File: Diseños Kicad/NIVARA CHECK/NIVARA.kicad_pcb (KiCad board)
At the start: 2 copper layers, 107 x 87.7 mm, 41 parts, among them J1 Screw_Terminal_01x02, J10 Screw_Terminal_01x02, J12 Screw_Terminal_01x04, J2 Screw_Terminal_01x02, J3 Screw_Terminal_01x04, J4 Screw_Terminal_01x02, J5 Screw_Terminal_01x02, J6 Screw_Terminal_01x06, J7 Screw_Terminal_01x03, J9 Screw_Terminal_01x02, K1 G2RL-1, K2 G2RL-1, Q1 NCV8402xST, Q3 NCV8402xST, Q4 NCV8402xST, Q5 NCV8402xST, U1 ESP32-S3-WROOM-1, U10 LTV-357TB, U12 LTV-357T, U13 LTV-357T, U14 LTV-357T, U15 LTV-357TB, U2 AP63200WU, U2 AP63203WU, U4 LTV-357TB, U5 LTV-357T, U7 LTV-357TB, U8 LTV-357TB, U9 LTV-357TB

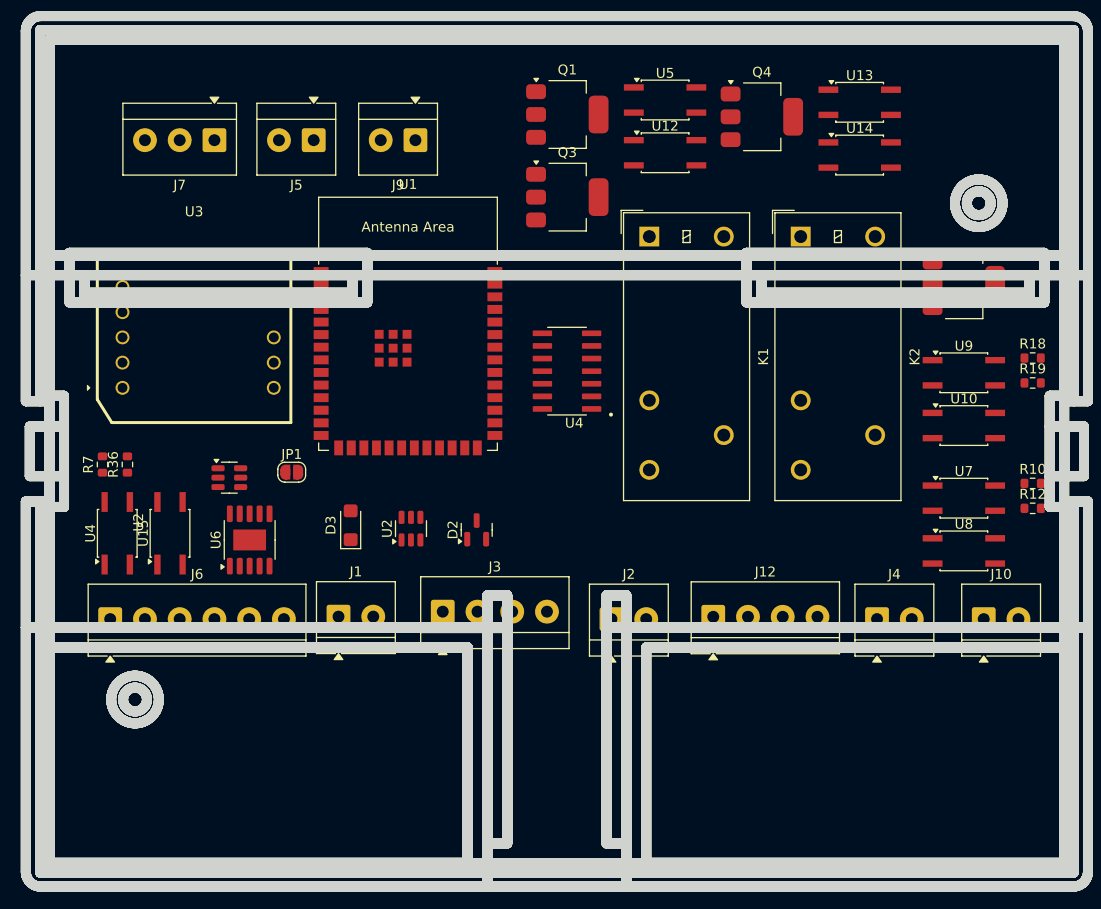
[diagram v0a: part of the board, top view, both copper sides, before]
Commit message: detallitos
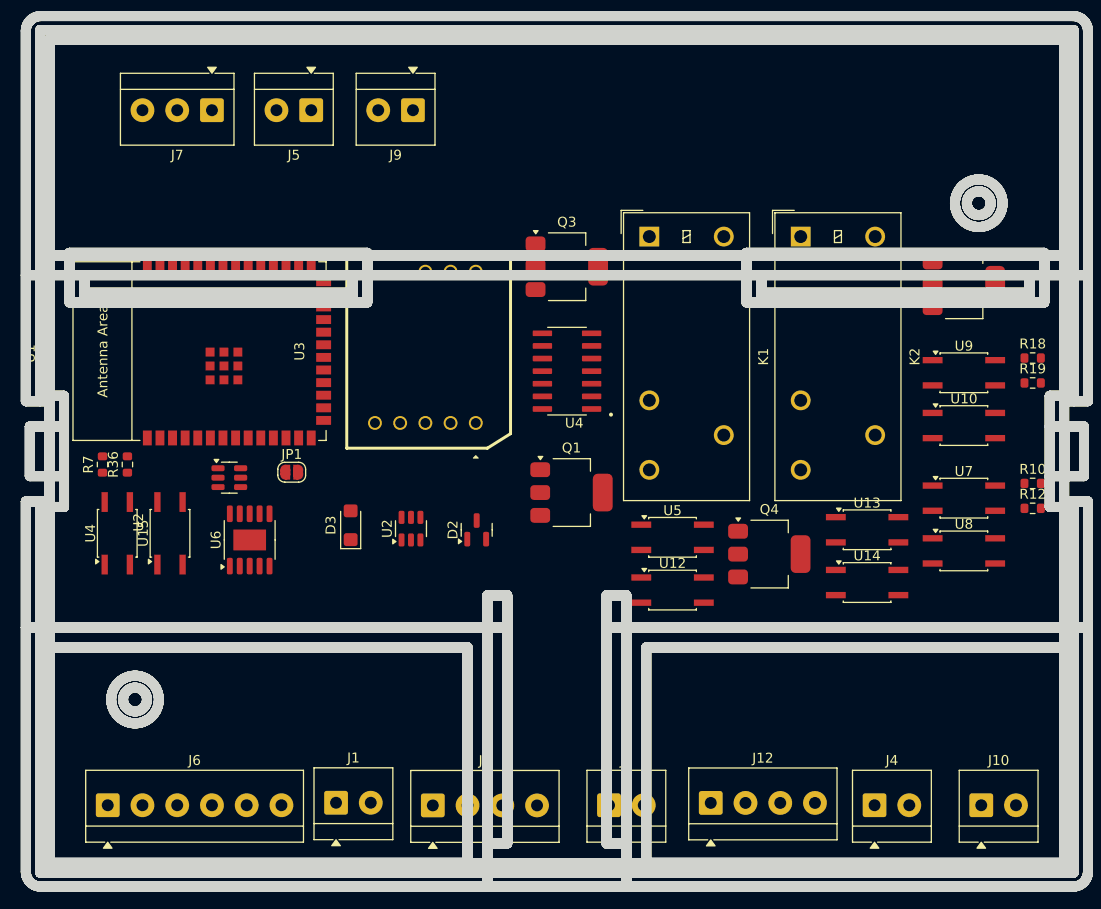
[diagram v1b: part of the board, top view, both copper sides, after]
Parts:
- moved U5 44.1 mm to (165.2, 83.0)
- moved Q4 44.1 mm to (174.9, 84.7)
- moved U12 44.1 mm to (165.2, 88.3)
- moved U13 43.1 mm to (184.8, 82.2)
- moved U14 43.1 mm to (184.8, 87.6)
- moved U3 41.7 mm to (148.8, 74.0), turned to 90 degrees
- moved Q1 38.1 mm to (155.0, 78.5)
- moved J3 19.5 mm to (141.0, 110.0)
- moved J1 18.8 mm to (131.2, 109.8)
- moved J10 18.8 mm to (196.2, 110.0)
- moved J12 18.8 mm to (169.0, 109.8)
- moved J2 18.8 mm to (158.8, 110.0)
- moved J4 18.8 mm to (185.5, 110.0)
- moved J6 18.8 mm to (108.2, 110.0)
- moved U1 18.0 mm to (120.5, 64.2), turned to 90 degrees
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
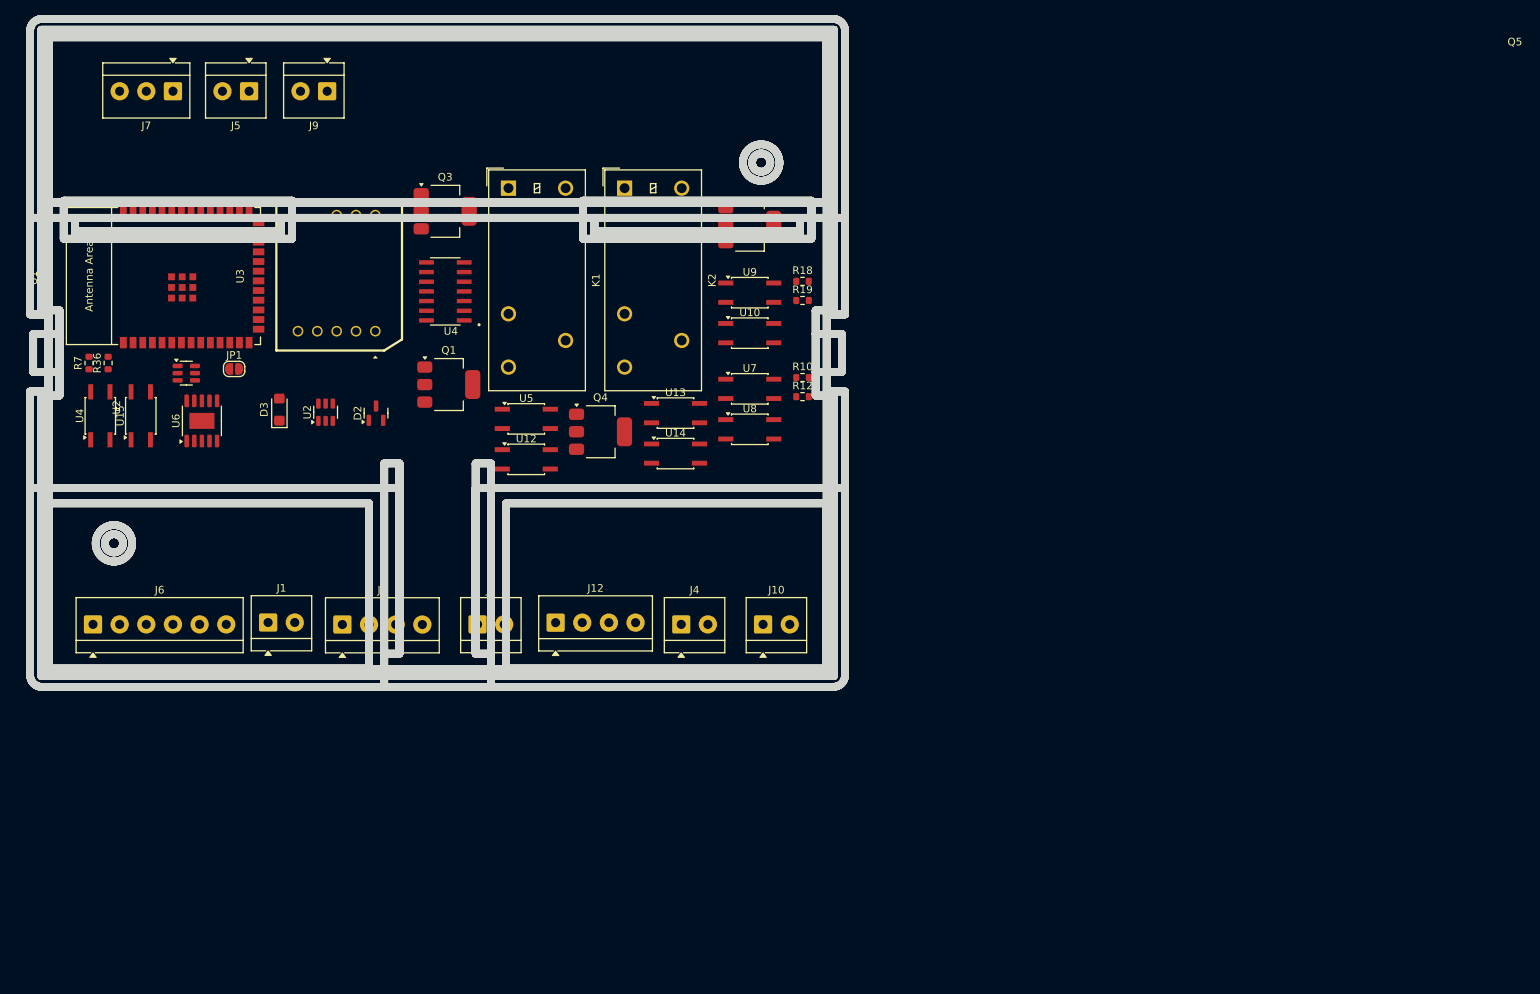
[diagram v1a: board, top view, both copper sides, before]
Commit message: YA AAAAAAAAAAAAAAAA
Detallitos sobre el dxf que estaba mal
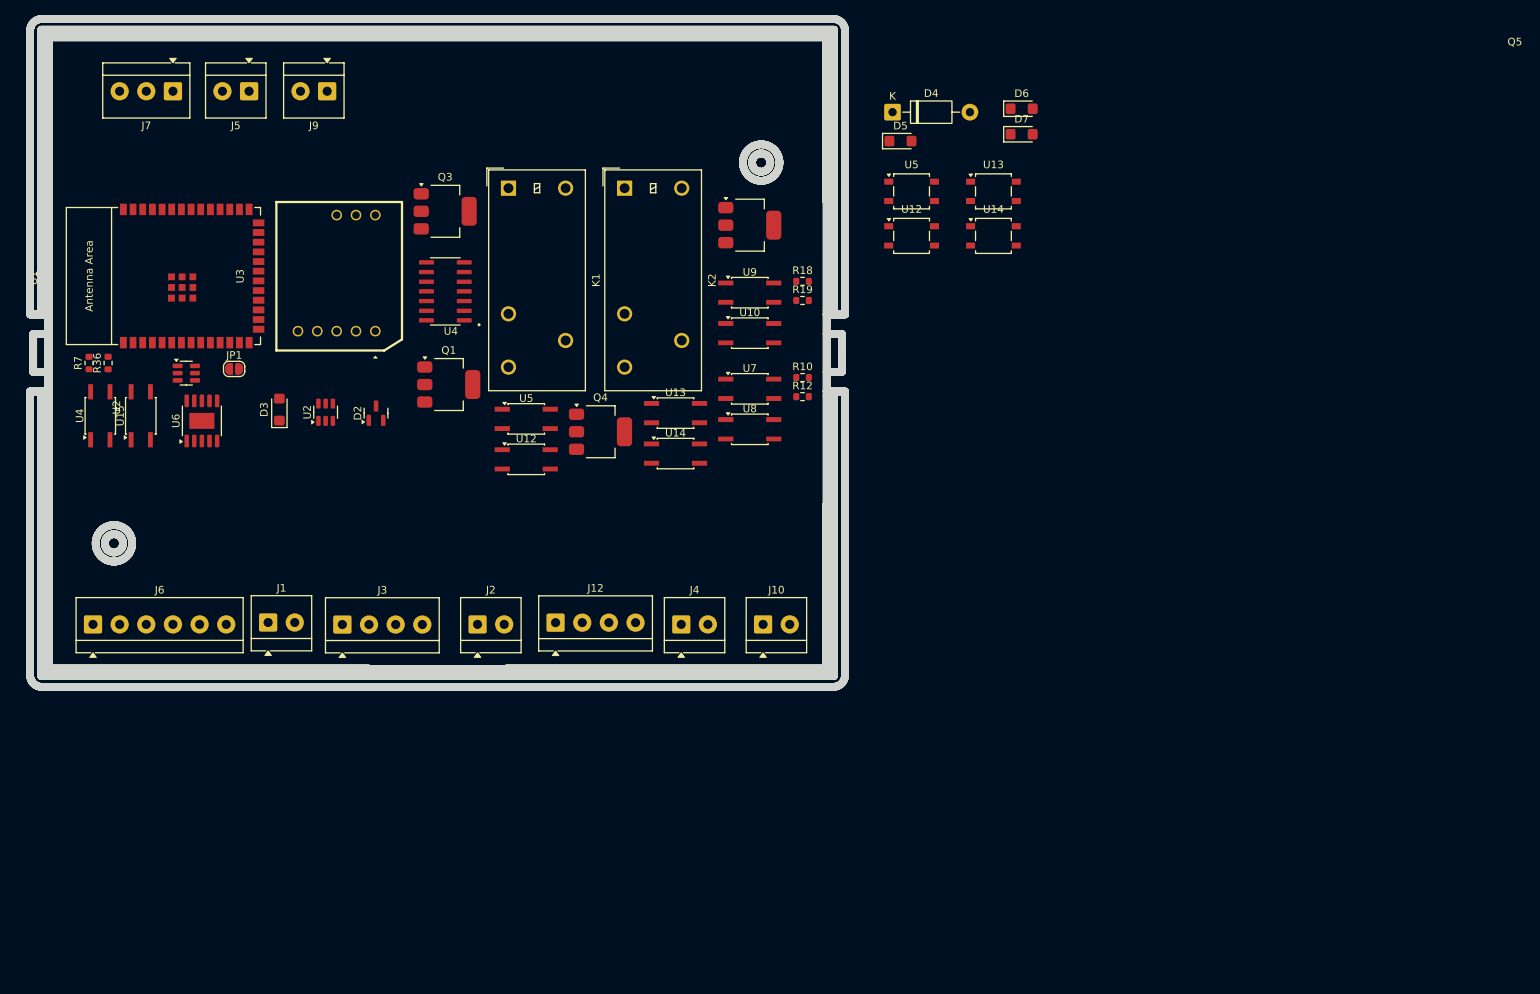
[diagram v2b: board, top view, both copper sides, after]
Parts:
- added D4: 1N4007, Diode_THT:D_DO-41_SOD81_P10.16mm_Horizontal, F.Cu at (213.2, 42.7)
- added D5: SMF24A, Diode_SMD:D_SMF, F.Cu at (214.3, 46.5)
- added D6: SMF24A, Diode_SMD:D_SMF, F.Cu at (230.2, 42.3)
- added D7: SMF24A, Diode_SMD:D_SMF, F.Cu at (230.2, 45.6)
- added U12: ~, Package_SO:SO-4_4.4x4.3mm_P2.54mm, F.Cu at (215.8, 59.0)
- added U13: ~, Package_SO:SO-4_4.4x4.3mm_P2.54mm, F.Cu at (226.5, 53.1)
- added U14: ~, Package_SO:SO-4_4.4x4.3mm_P2.54mm, F.Cu at (226.5, 59.0)
- added U5: ~, Package_SO:SO-4_4.4x4.3mm_P2.54mm, F.Cu at (215.8, 53.1)
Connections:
- J12 pad 3: /NIVARA_BOARD/mA_AOUTPUT- -> unconnected-(J12-Pin_3-Pad3)
- J6 pad 1: /NIVARA_BOARD/RL1_COM -> /NIVARA_BOARD/RL1_OUTPUT_NO
- J6 pad 5: /NIVARA_BOARD/RL1_COM -> /NIVARA_BOARD/RL2_OUTPUT_NC
- JP1 pad 1: Net-(JP1-A) -> Net-(D6-A1)
- K1 pad 12: /NIVARA_BOARD/RL1_COM -> /NIVARA_BOARD/RL2_OUTPUT_NC
- K2 pad 14: /NIVARA_BOARD/RL1_COM -> /NIVARA_BOARD/RL1_OUTPUT_NO
- U1 pad 12: unconnected-(U1-GPIO8/TOUCH8/ADC1_CH7/SUBSPICS1-Pad12) -> /NIVARA_BOARD/PNP_IN_Mod/NPN_Output0
- U1 pad 16: unconnected-(U1-GPIO46-Pad16) -> /NIVARA_BOARD/~{TRANSMIT}/RECEIVE
- U1 pad 17: unconnected-(U1-GPIO9/TOUCH9/ADC1_CH8/FSPIHD/SUBSPIHD-Pad17) -> /NIVARA_BOARD/PNP_IN_Mod/NPN_Output1
- U1 pad 18: unconnected-(U1-GPIO10/TOUCH10/ADC1_CH9/FSPICS0/FSPIIO4/SUBSPICS0-Pad18) -> /NIVARA_BOARD/DRY_INPUT_INTERFAZ/DRY_OUT0
- U1 pad 23: unconnected-(U1-GPIO21-Pad23) -> /NIVARA_BOARD/DRY_INPUT_INTERFAZ/DRY_OUT1
- U1 pad 24: unconnected-(U1-GPIO47/SPICLK_P/SUBSPICLK_P_DIFF-Pad24) -> /NIVARA_BOARD/RS485_INTERFAZ/UART_TX
- U1 pad 25: unconnected-(U1-GPIO48/SPICLK_N/SUBSPICLK_N_DIFF-Pad25) -> /NIVARA_BOARD/RS485_INTERFAZ/UART_RX
- U1 pad 26: unconnected-(U1-GPIO45-Pad26) -> /NIVARA_BOARD/NPN_OUT_INTERFAZ/NPN_EN1
- U1 pad 28: unconnected-(U1-SPIIO6/GPIO35/FSPID/SUBSPID-Pad28) -> /NIVARA_BOARD/VOLTAGE_AOUT_INTERFAZ/SEL
- U1 pad 29: unconnected-(U1-SPIIO7/GPIO36/FSPICLK/SUBSPICLK-Pad29) -> /NIVARA_BOARD/~{RUN}/STOP
- U1 pad 31: unconnected-(U1-GPIO38/FSPIWP/SUBSPIWP-Pad31) -> /NIVARA_BOARD/NPN_OUT_INTERFAZ/NPN_EN0
- U1 pad 36: /NIVARA_BOARD/RS485_INTERFAZ/UART_RX -> unconnected-(U1-U0RXD/GPIO44/CLK_OUT2-Pad36)
- U1 pad 37: /NIVARA_BOARD/RS485_INTERFAZ/UART_TX -> unconnected-(U1-U0TXD/GPIO43/CLK_OUT1-Pad37)
- U1 pad 4: unconnected-(U1-GPIO4/TOUCH4/ADC1_CH3-Pad4) -> /NIVARA_BOARD/32V_AIN_INTERFAZ/32V_ADC
- U1 pad 5: unconnected-(U1-GPIO5/TOUCH5/ADC1_CH4-Pad5) -> /NIVARA_BOARD/10V_AIN_INTERFAZ/10V_ADC
- U1 pad 6: unconnected-(U1-GPIO6/TOUCH6/ADC1_CH5-Pad6) -> /NIVARA_BOARD/PNP_OUT_INTERFAZ/PNP_EN0
- U1 pad 7: unconnected-(U1-GPIO7/TOUCH7/ADC1_CH6-Pad7) -> /NIVARA_BOARD/PNP_OUT_INTERFAZ/PNP_EN1
- U1 pad 8: unconnected-(U1-GPIO15/U0RTS/ADC2_CH4/XTAL_32K_P-Pad8) -> /NIVARA_BOARD/VOLTAGE_AOUT_INTERFAZ/SCLK
- U1 pad 9: unconnected-(U1-GPIO16/U0CTS/ADC2_CH5/XTAL_32K_N-Pad9) -> /NIVARA_BOARD/VOLTAGE_AOUT_INTERFAZ/SCLK
- U6 pad 1: unconnected-(U6-SCLK-Pad1) -> /NIVARA_BOARD/VOLTAGE_AOUT_INTERFAZ/SCLK
- U6 pad 2: unconnected-(U6-SDA-Pad2) -> /NIVARA_BOARD/VOLTAGE_AOUT_INTERFAZ/SCLK
- U6 pad 8: unconnected-(U6-IOUT-Pad8) -> Net-(U6-IOUT)
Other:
- outline, holes or cut-outs redrawn

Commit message: bueno avance v45352
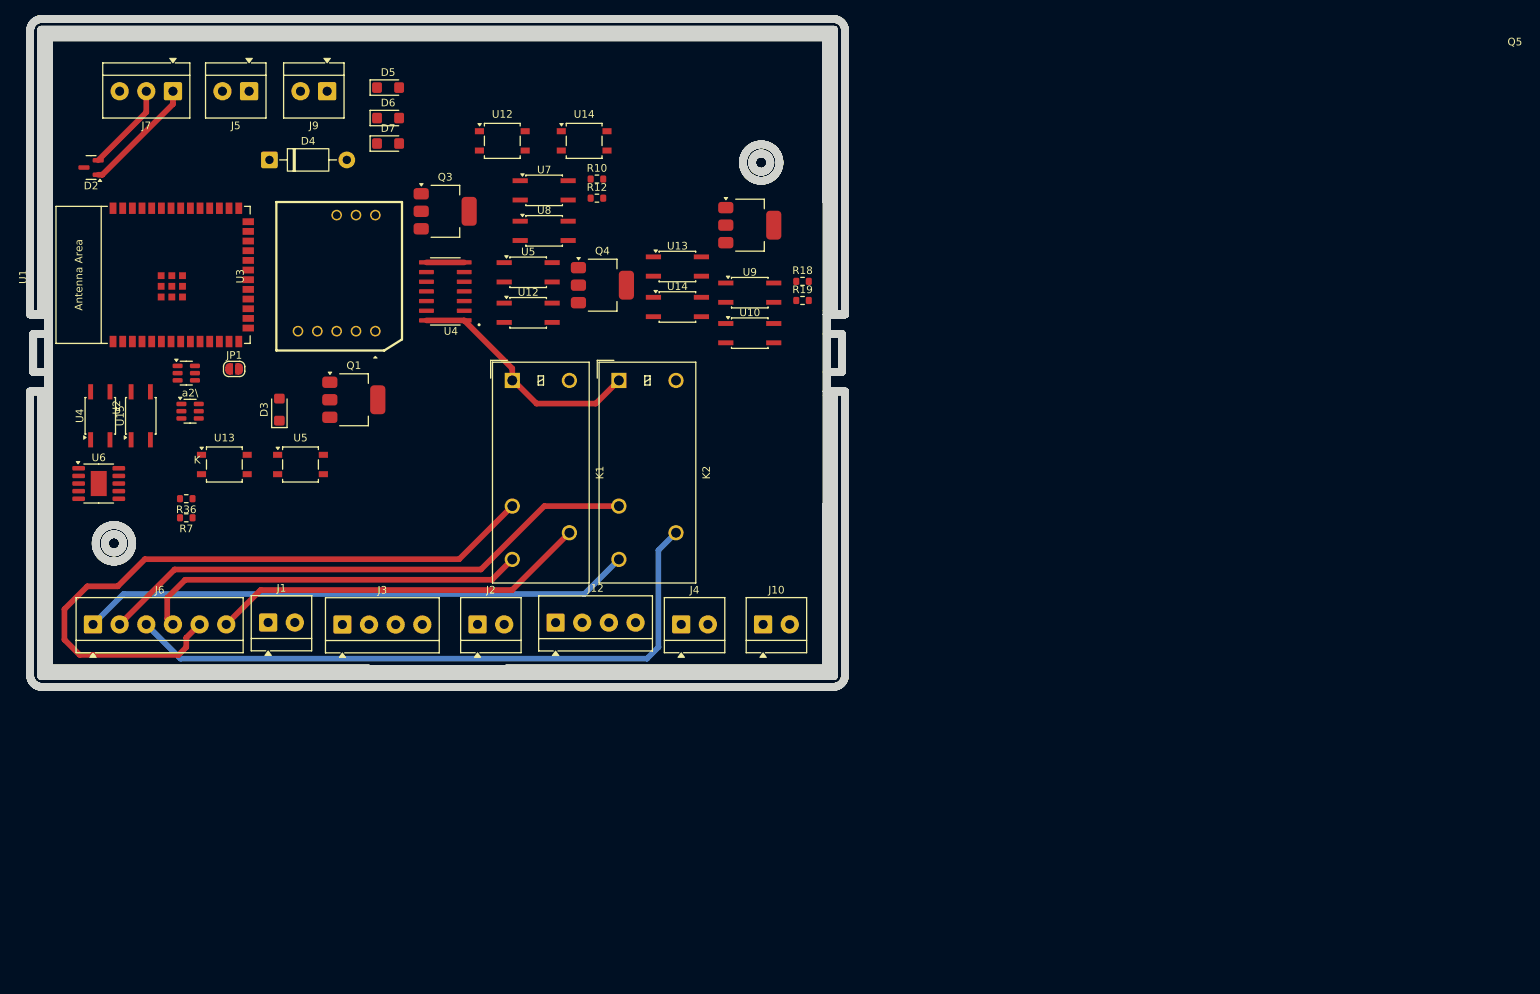
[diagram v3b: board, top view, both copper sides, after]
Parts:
- moved U13 107.2 mm to (125.5, 89.0)
- moved U5 87.9 mm to (135.5, 89.0)
- moved D6 83.2 mm to (147.0, 43.5)
- moved D7 83.2 mm to (147.0, 46.9)
- moved D4 82.1 mm to (131.4, 49.0)
- moved D5 67.7 mm to (147.0, 39.5)
- moved U12 55.2 mm to (162.0, 46.5)
- moved U14 55.2 mm to (172.8, 46.5)
- moved D2 49.4 mm to (108.0, 50.0), turned to 180 degrees
- moved R10 37.5 mm to (174.4, 51.5)
- moved R12 37.5 mm to (174.4, 54.0)
- moved U7 37.5 mm to (167.5, 53.0)
- moved U8 37.5 mm to (167.5, 58.3)
- moved K2 25.3 mm to (177.3, 78.0)
- moved K1 25.3 mm to (163.3, 78.0)
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- renumbered U2 to a2\
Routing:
- net /NIVARA_BOARD/RL2_OUTPUT_NC: track 0.00 -> 89.4 mm
- net /NIVARA_BOARD/RL1_COM: track 0.00 -> 85.7 mm
- net /NIVARA_BOARD/RL1_OUTPUT_NO: track 0.00 -> 72.6 mm
- net /NIVARA_BOARD/RL1_OUTPUT_NC: track 0.00 -> 72.0 mm
- net /NIVARA_BOARD/RL2_OUTPUT_NO: track 0.00 -> 51.6 mm
- net /NIVARA_BOARD/RL2_COM: track 0.00 -> 50.0 mm
- net VCC: track 0.00 -> 36.9 mm
- net /NIVARA_BOARD/RS485_A: track 0.00 -> 15.3 mm
- net /NIVARA_BOARD/RS485_B: track 0.00 -> 11.7 mm
